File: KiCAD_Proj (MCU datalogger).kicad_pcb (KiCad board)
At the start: 2 copper layers, 52.3 x 34.7 mm, 31 parts, among them J1 Conn_01x04_Pin, J2 Conn_01x09_Pin, J3 Conn_01x04_Pin, J4 Conn_02x03_Counter_Clockwise, U1 24LC1025-I_SM, U2 DS1337S_, U3 24LC1025-I_SM, U4 ATMEGA328P-AU, Y1 32.768 KHz, Y2 16MHz

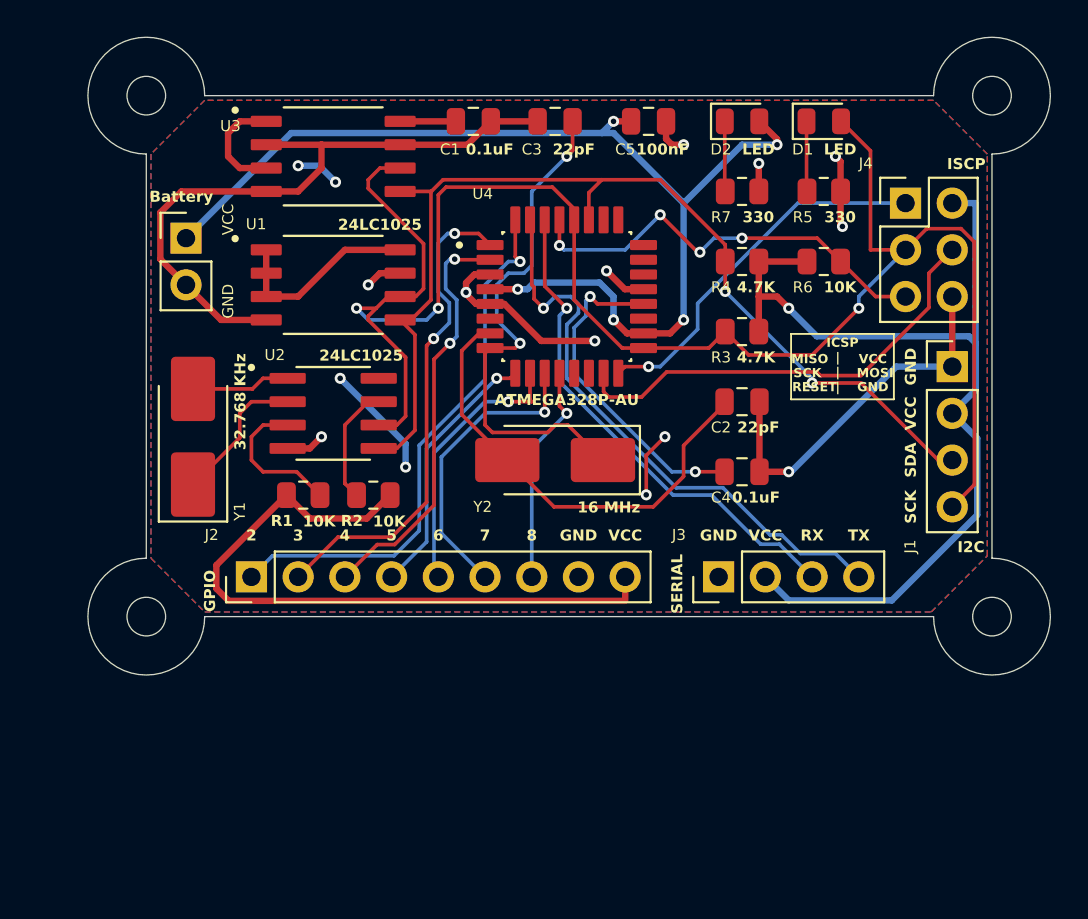
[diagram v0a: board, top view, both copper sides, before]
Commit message: Updated the pcb.
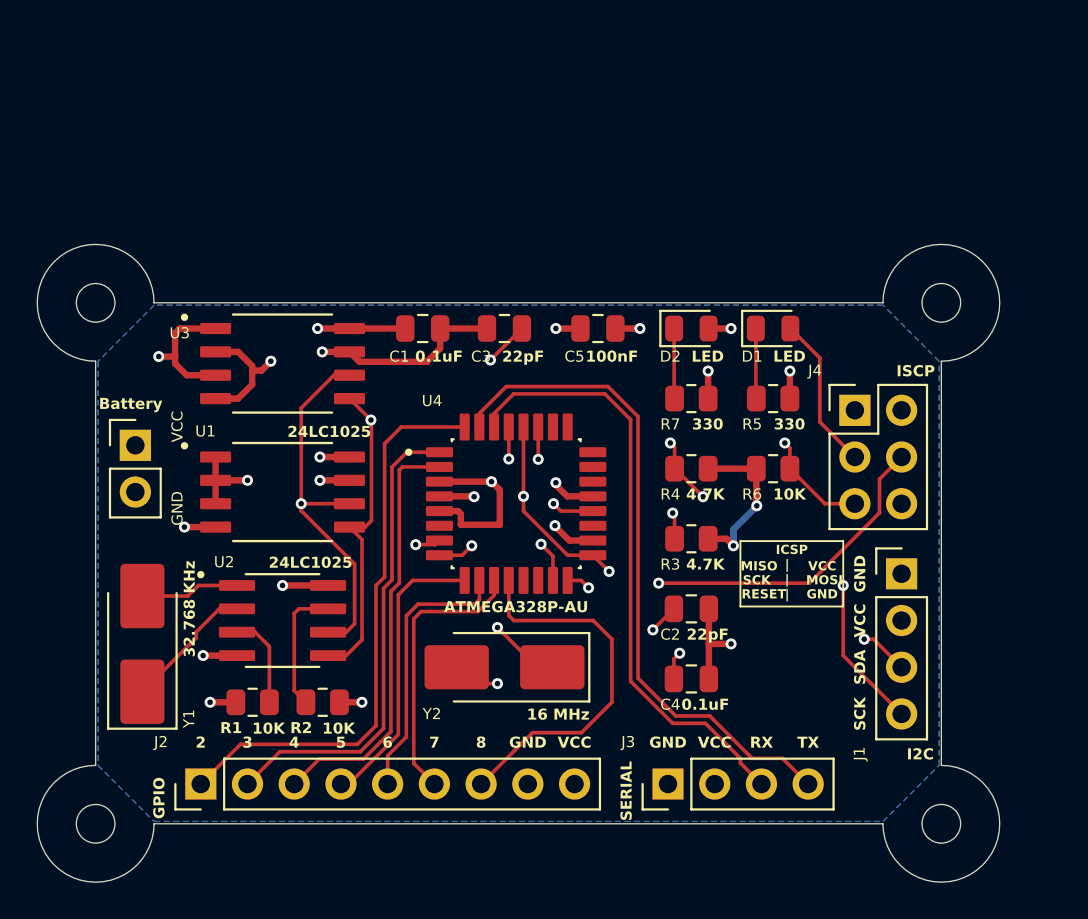
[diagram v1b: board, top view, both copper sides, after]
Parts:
- moved C3 11.6 mm to (110.9, 90.0)
- moved C5 11.6 mm to (116.0, 90.0)
- moved D1 11.6 mm to (125.5, 90.0)
- moved D2 11.6 mm to (121.1, 90.0)
- moved G*** 11.6 mm to (98.5, 98.9)
- moved J3 11.6 mm to (119.8, 114.8)
- moved R5 11.6 mm to (125.5, 93.8)
- moved R7 11.6 mm to (121.1, 93.8)
- moved C1 11.6 mm to (106.5, 90.0)
- moved J2 11.6 mm to (94.4, 114.8)
- moved U1 11.6 mm to (98.8, 98.9)
- moved U2 11.6 mm to (98.8, 105.9)
- moved U3 11.6 mm to (98.8, 91.9)
- moved BT1 11.6 mm to (90.8, 96.4)
- moved C2 11.6 mm to (121.1, 105.2)
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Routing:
- net /Vcc: track 178.4 -> 43.8 mm, vias 10 -> 13
- net GND: track 84.2 -> 43.6 mm, vias 12 -> 11
- net /SCK: track 97.6 -> 86.6 mm, vias 3 -> 5
- net /D8: track 12.0 -> 20.4 mm, vias 1 -> 0
- net /RX: track 27.6 -> 33.0 mm, vias 1 -> 0
- net /TX: track 32.1 -> 36.5 mm, vias 1 -> 0
- net Net-(U4-PB7): track 28.4 -> 25.2 mm, vias 2 -> 3
- net Net-(U2-~{INTA}): track 8.02 -> 5.12 mm
- net /SDA: track 57.4 -> 55.1 mm, vias 2 -> 5
- net /MOSI: track 24.7 -> 26.6 mm, vias 0 -> 2
- net /D5: track 14.3 -> 15.8 mm, vias 1 -> 0
- net Net-(U4-AREF): track 18.0 -> 19.4 mm
- net /D2: track 29.8 -> 31.1 mm, vias 1 -> 0
- net /D7: track 16.2 -> 15.2 mm, vias 1 -> 0
- net Net-(U4-PB6): track 25.5 -> 24.6 mm, vias 0 -> 3
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- added copper zone on In1.Cu, net /Vcc
- removed copper zone on F.Cu, net /Vcc
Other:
- copper layers 2 -> 4
